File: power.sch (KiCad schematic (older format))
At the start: 8 parts, among them U24 TLV62569P

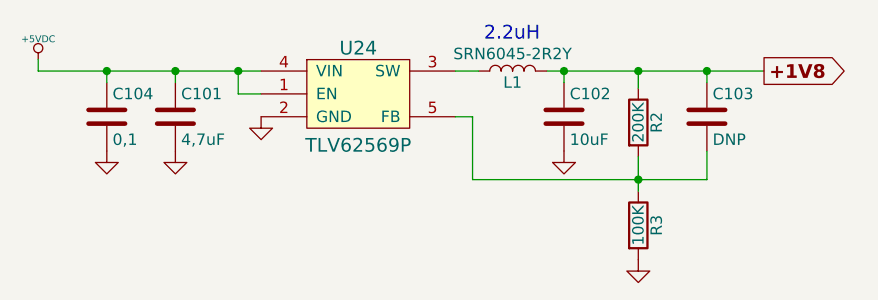
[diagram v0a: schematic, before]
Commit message: Update 1V8 PSU
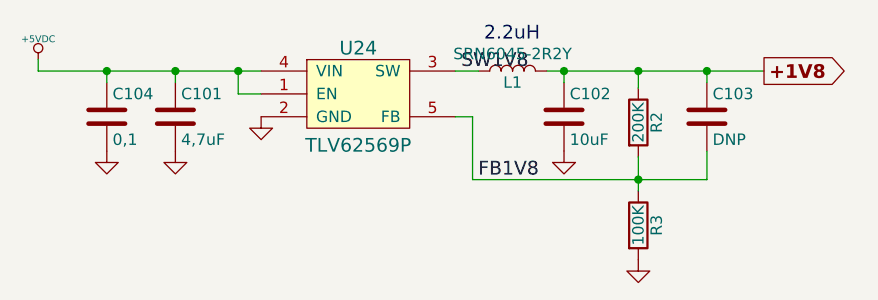
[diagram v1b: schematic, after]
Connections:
- net SW1V8: now reaches L1.1, U24.3 (SW)
- net FB1V8: now reaches C103.2, R2.2, R3.1, U24.5 (FB)
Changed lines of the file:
@@
 $EndComp
 $Comp
-L GND #PWR148
+L GND #PWR0147
 U 1 1 588CA667
 P 5000 3850
-F 0 "#PWR148" H 5000 3600 50  0001 C CNN
+F 0 "#PWR0147" H 5000 3600 50  0001 C CNN
 F 1 "GND" H 5000 3700 50  0001 C CNN
 F 2 "" H 5000 3850 50  0000 C CNN
@@
 Connection ~ 4625 3650
 $Comp
-L GND #PWR150
+L GND #PWR0148
 U 1 1 588CA72B
 P 4625 4000
-F 0 "#PWR150" H 4625 3750 50  0001 C CNN
+F 0 "#PWR0148" H 4625 3750 50  0001 C CNN
 F 1 "GND" H 4625 3850 50  0001 C CNN
 F 2 "" H 4625 4000 50  0000 C CNN
@@
 	6650 4025 6650 4175
 $Comp
-L GND #PWR152
+L GND #PWR0149
 U 1 1 588CB06D
 P 6650 4475
-F 0 "#PWR152" H 6650 4225 50  0001 C CNN
+F 0 "#PWR0149" H 6650 4225 50  0001 C CNN
 F 1 "GND" H 6650 4325 50  0001 C CNN
 F 2 "" H 6650 4475 50  0000 C CNN
@@
 $EndComp
 $Comp
-L GND #PWR151
+L GND #PWR0150
 U 1 1 588CB1AB
 P 6325 4000
-F 0 "#PWR151" H 6325 3750 50  0001 C CNN
+F 0 "#PWR0150" H 6325 3750 50  0001 C CNN
 F 1 "GND" H 6325 3850 50  0001 C CNN
 F 2 "" H 6325 4000 50  0000 C CNN
@@
 +1V8
 $Comp
-L +5VDC #PWR147
+L +5VDC #PWR0151
 U 1 1 588CF502
 P 4025 3600
-F 0 "#PWR147" H 4125 3650 20  0001 C CNN
+F 0 "#PWR0151" H 4125 3650 20  0001 C CNN
 F 1 "+5VDC" H 4025 3690 30  0000 C CNN
 F 2 "" H 4025 3600 60  0000 C CNN
@@
 Connection ~ 4325 3650
 $Comp
-L GND #PWR149
+L GND #PWR0152
 U 1 1 588D28B5
 P 4325 4000
-F 0 "#PWR149" H 4325 3750 50  0001 C CNN
+F 0 "#PWR0152" H 4325 3750 50  0001 C CNN
 F 1 "GND" H 4325 3850 50  0001 C CNN
 F 2 "" H 4325 4000 50  0000 C CNN
@@
 Text Notes 5975 3525 0    60   ~ 0
 2.2uH
+Text Label 5950 4125 0    60   ~ 0
+FB1V8
+Text Label 5875 3650 0    60   ~ 0
+SW1V8
 $EndSCHEMATC
